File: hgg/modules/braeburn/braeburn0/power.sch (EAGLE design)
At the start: 54 parts, among them IC1 7812TV, IC2 7805TV, IC3 7805TV, IC4 ATMEGA48/88/168-AU

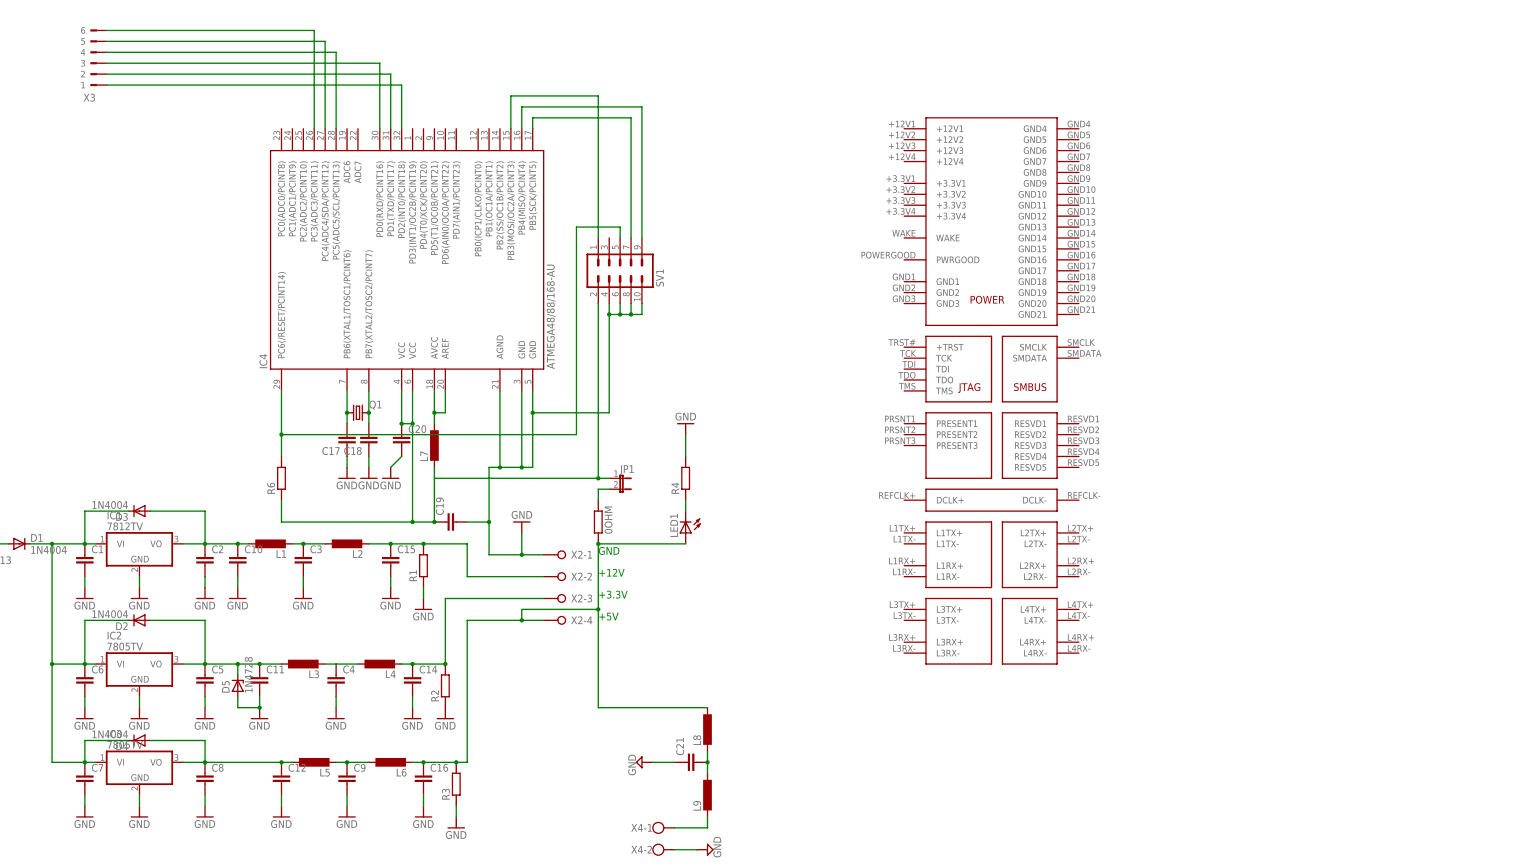
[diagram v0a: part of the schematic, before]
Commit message: new release of braeburn board file
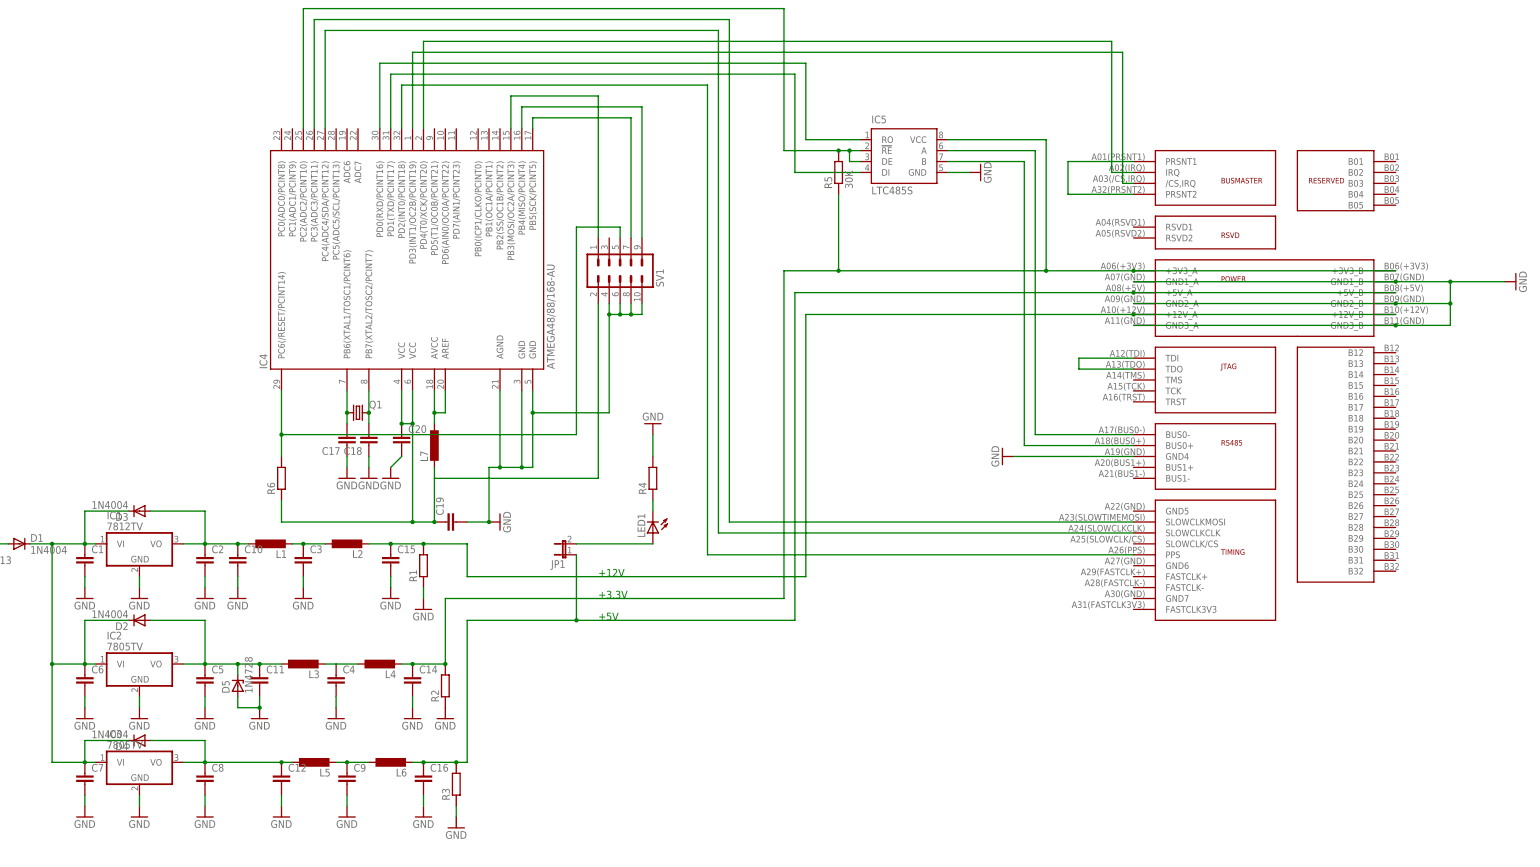
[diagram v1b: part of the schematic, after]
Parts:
- removed 0OHM: (no value), rcl:R-EU_0411/15
- removed C21: (no value), rcl:C-EUC0805
- removed L8, L9: (no value), rcl:L-EU0207/5V
- removed X2: (no value), con-wago-508:W237-04P
- removed X3: (no value), con-weidmueller-sl35:180G-6
- removed X4: (no value), con-wago-500:W237-102
- added IC5: LTC485S, linear-technology:LTC485S
- added R5: 30K, rcl:R-EU_R0603
- C17, C18, C19, C20: device rcl:C-EUC0805 -> rcl:C-EUC0603
- R4: device rcl:R-EU_R2012 -> rcl:R-EU_R0603
- R6: device resistor:R-EU_R0805 -> resistor:R-EU_R0603
- U$1: value FRIENDSHIPEDGECONNECTOR -> FRIENDSHIPCONNECTOR; device hgg:FRIENDSHIPEDGECONNECTOR -> hgg:FRIENDSHIPCONNECTOR
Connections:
- new net N$31: C16.1, JP1.1, L6.2, R3.2, U$1.+5V_A, U$1.+5V_B
- new net N$32: IC4.PC2(ADC2/PCINT10), IC5.!RE, IC5.DE, R5.2
- new net N$33: IC4.PD3(INT1/OC2B/PCINT19), U$1./CS,IRQ
- new net N$34: IC4.PD4(T0/XCK/PCINT20), U$1.IRQ
- net GND: now also IC5.GND, U$1.GND1_A, U$1.GND1_B, U$1.GND2_A, U$1.GND2_B, U$1.GND3_A, U$1.GND3_B, U$1.GND4; no longer C21.1, X2-1.KL, X4-2.KL
- net N$10: now also IC5.VCC, R5.1, U$1.+3V3_A, U$1.+3V3_B; no longer X2-3.KL
- net N$11: now also IC5.A, U$1.BUS0-; no longer 0OHM.2, C16.1, L6.2, L8.1, LED1.A, R3.2, X2-4.KL
- net N$20: now also U$1.PPS; no longer X3.1
- net N$21: now also IC5.DI; no longer X3.2
- net N$22: now also IC5.B, U$1.BUS0+; no longer IC4.PD0(RXD/PCINT16), X3.3
- net N$23: now also U$1.PRSNT1, U$1.PRSNT2; no longer IC4.PC5(ADC5/SCL/PCINT13), X3.4
- net N$24: now also U$1.SLOWCLKCLK; no longer X3.5
- net N$25: now also U$1.SLOWCLKMOSI; no longer X3.6
- net N$27: no longer JP1.1
- net N$28: now also U$1.+12V_A, U$1.+12V_B; no longer X2-2.KL
- net N$29: now also U$1.TDI, U$1.TDO; no longer C21.2, L8.2, L9.1
- net N$30: now also IC4.PD0(RXD/PCINT16), IC5.RO; no longer L9.2, X4-1.KL
- net N$9: now also LED1.A; no longer 0OHM.1
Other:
- note removed: "GND"
- moved on the sheet: JP1, LED1, R4

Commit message: initial version of design update
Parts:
- removed C16: (no value), capacitor-wima:C5/7.2
- removed D5: 1N4728, diode:1N4728
- removed IC2, IC3: 7805TV, linear:7805TV
- removed L2, L4, L6: (no value), resistor:L-EU0207/5V
- added LED2, LED4: GM5BW96385A, led:GM5BW96385A
- added R10, R11, R12, R13, R14, R15, R16, R17, R18, R7, R8, R9: (no value), rcl:R-EU_R0603
- added R19, R20, R21: (no value), rcl:R-EU_0207/15
- added R22: PTC-SOD70, ptc-ntc:PTC-SOD70
- added R23, R24, R25: 2k, rcl:R-EU_R0603
- added U$2, U$3, U$4: AP1084, hgg:AP1084
- C13: value (none) -> 2000u
- C14: value (none) -> 100n; device capacitor-wima:C5/7.2 -> rcl:C-EUC0603
- C15: device capacitor-wima:C5/7.2 -> rcl:C-EUC0603
- C17, C18: value (none) -> 22n
- C19: value (none) -> 2n2
- C20: value (none) -> 100n
- IC1: value 7812TV -> LM324D; device linear:7812TV -> linear:LM324D
- L7: value (none) -> 33u
- R5: value 30K -> 10k
- R6: value (none) -> 10k
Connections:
- net N$11 renamed BUS0-
- net N$14 renamed RST
- net N$22 renamed BUS0+
- net N$33 renamed /CS
- net N$34 renamed IRQ
- removed net N$31: C16.1, JP1.1, L6.2, R3.2, U$1.+5V_A, U$1.+5V_B
- new net 12V: R16.1, R21.2, U$1.+12V_A, U$1.+12V_B
- new net 12VIN: C9.1, L5.2, R17.1, R21.1, R3.2
- new net 3V3: R19.2, R7.1, U$1.+3V3_A, U$1.+3V3_B
- new net 3V3IN: C3.1, L1.2, R1.2, R19.1, R9.1
- new net LED1: IC4.PD5(T1/OC0B/PCINT21), LED2.A
- new net LED2: IC4.PD6(AIN0/OC0A/PCINT22), LED4.A
- new net N$11: IC1B.OUT, R13.2
- new net N$14: IC1B.-IN, R12.2, R14.2
- new net N$22: IC1B.+IN, R11.2, R13.1
- new net N$26: IC1C.+IN, R15.1, R16.2
- new net N$36: LED2.C, R24.1
- new net N$37: LED4.C, R25.1
- new net TEMP1: IC4.ADC6, R22.2, R23.2
- new net VCC: C14.2, C15.2, C19.1, C20.1, IC1P.V+, IC4.VCC@1, IC4.VCC@2, IC5.VCC, JP1.1, L7.2, R11.1, R20.2, R23.1, R5.1, R6.1, SV1.2, U$1.+5V_A, U$1.+5V_B
- new net VCCIN: C4.1, L3.2, R12.1, R2.2, R20.1
- net GND: now also C14.1, C15.1, IC1P.V-, R10.1, R14.1, R18.1, R22.1, R24.2, R25.2, U$2.GND, U$3.GND, U$4.GND; no longer C14.2, C15.2, C16.2, D5.A, IC1.GND, IC2.GND, IC3.GND
- net N$1: now also U$2.VIN, U$3.VIN, U$4.VIN; no longer IC1.VI, IC2.VI, IC3.VI
- net N$10: now also IC1A.OUT, R8.2; no longer C14.1, IC5.VCC, L4.2, R2.2, R5.1, U$1.+3V3_A, U$1.+3V3_B
- net N$27: now also IC1C.OUT, R15.2; no longer C19.1, C20.1, IC4.VCC@1, IC4.VCC@2, L7.2, R6.1, SV1.2
- net N$28: now also IC1C.-IN, R17.2, R18.2; no longer C15.1, L2.2, R1.2, U$1.+12V_A, U$1.+12V_B
- net N$3: now also U$4.VOUT; no longer IC3.VO
- net N$4: now also U$3.VOUT; no longer D5.C, IC2.VO
- net N$5: now also U$2.VOUT; no longer IC1.VO
- net N$6: now also IC4.PC1(ADC1/PCINT9), U$1.SLOWCLK/CS; no longer C9.1, L5.2, L6.1
- net N$7: now also IC1A.-IN, R10.2, R9.2; no longer C4.1, L3.2, L4.1
- net N$8: now also IC1A.+IN, R7.2, R8.1; no longer C3.1, L1.2, L2.1
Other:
- note removed: "+12V"
- note removed: "+3.3V"
- note removed: "+5V"
- moved on the sheet: C1, C10, C11, C12, C13, C14, C15, C17, C18, C19, C2, C20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
